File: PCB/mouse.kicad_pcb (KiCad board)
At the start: 2 copper layers, 45 x 45 mm, 38 parts, among them J1 Conn_01x05_Shielded, J2 Conn_01x04_MountingPin, J3 Bat, J4 Conn_01x12, J5 Conn_01x12, SW1 SW_Push, U2 nice_nano

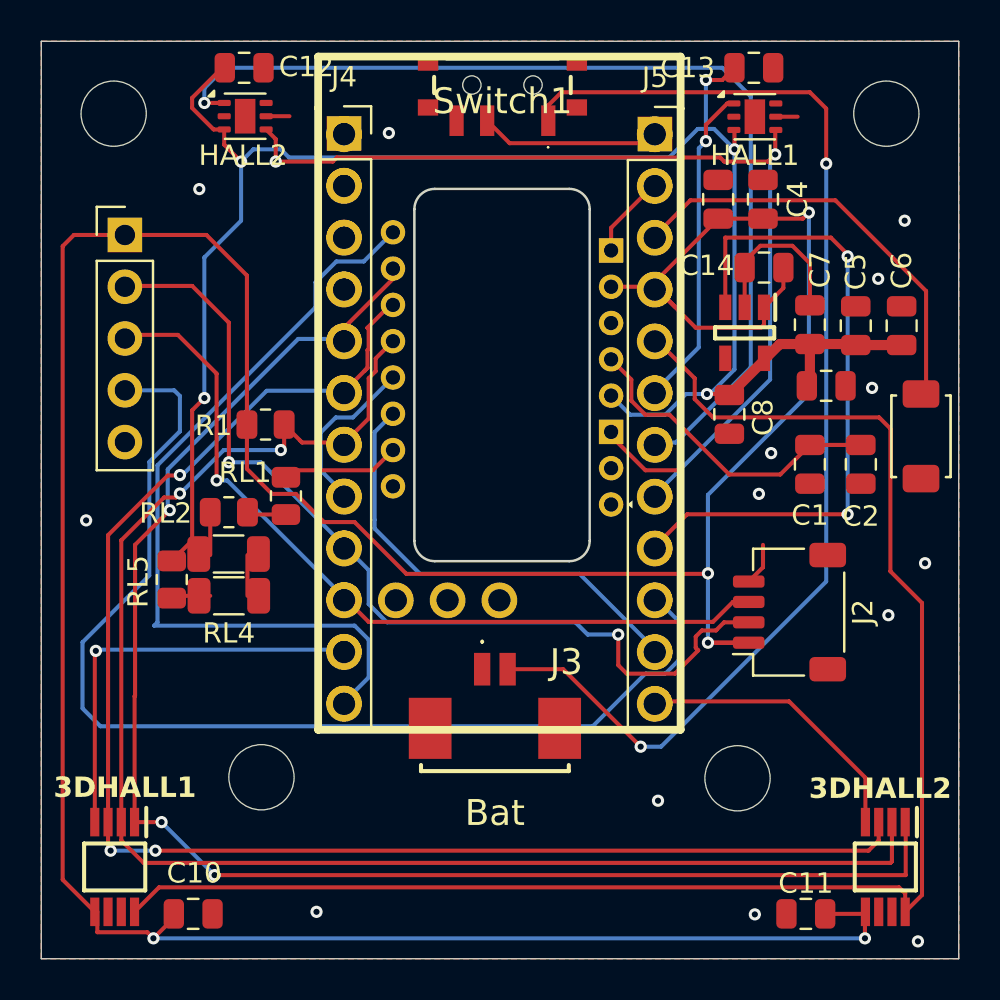
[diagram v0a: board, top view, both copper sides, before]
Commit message: bk
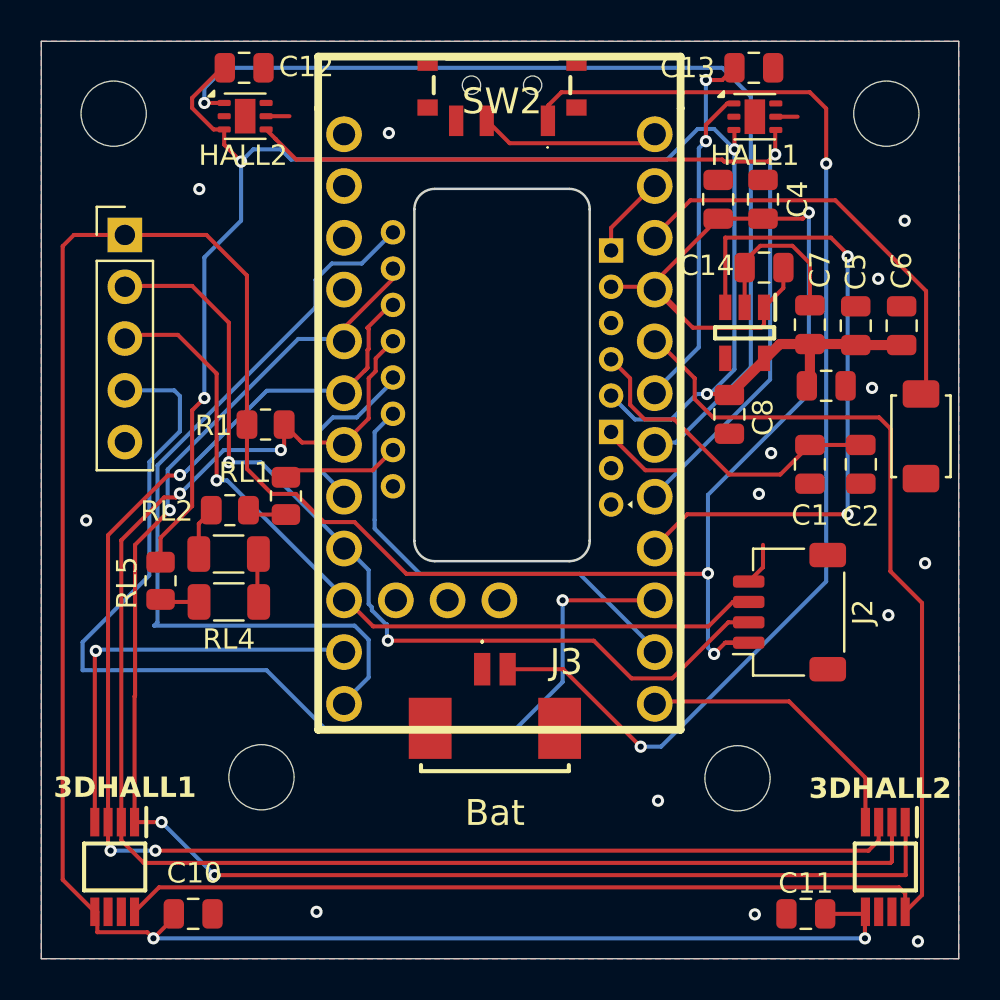
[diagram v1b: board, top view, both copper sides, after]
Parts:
- removed J4, J5: Conn_01x12, Connector_PinSocket_2.54mm:PinSocket_1x12_P2.54mm_Vertical
- removed Switch1: SSSS811101, SSSS811101:SSSS811101
- added SW2: SW_DPDT_x2, SSSS811101:SSSS811101, F.Cu at (183.6, 79.8)
- moved RL5 0.55 mm to (166.8, 104.2)
- moved RL4 0.30 mm to (170.2, 105.2)
- moved RL2 0.11 mm to (170.2, 100.7)
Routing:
- net INT: track 54.6 -> 52.5 mm, vias 0 -> 1
- net Left_control: track 47.3 -> 46.5 mm, vias 2 -> 1
- net SDA: track 46.0 -> 45.2 mm
- net 1.9v: track 89.2 -> 89.8 mm
